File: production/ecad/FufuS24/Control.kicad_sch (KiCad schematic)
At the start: 28 parts, among them J14 691137710004, J15 691137710004, J16 691137710004, J2 Conn_01x02, U1 RP2040, U2 W25Q128JVS

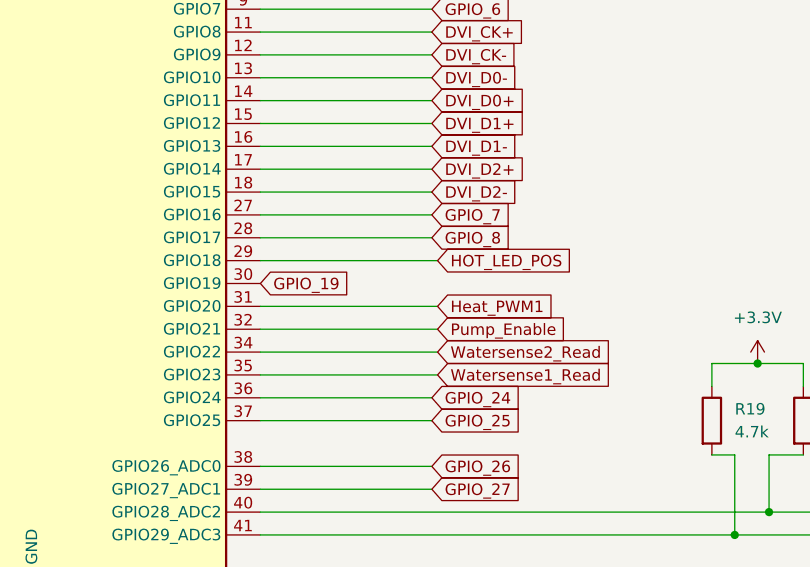
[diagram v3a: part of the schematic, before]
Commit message: changes
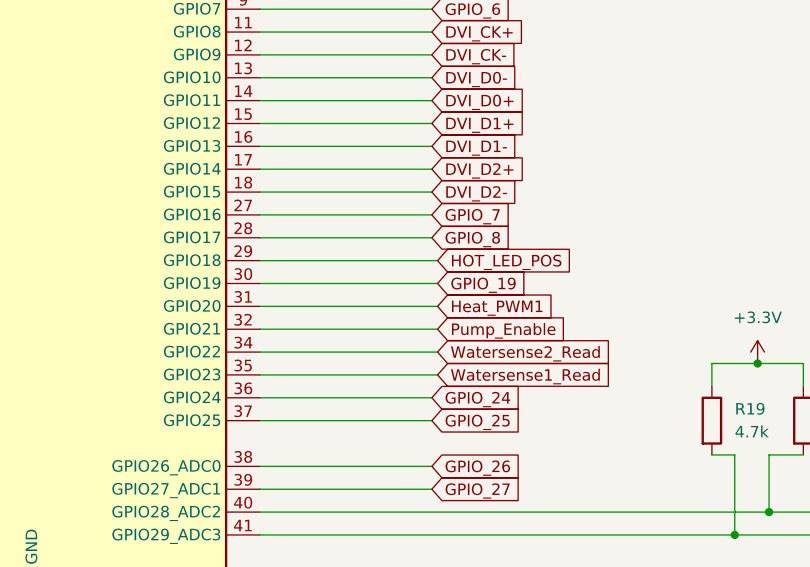
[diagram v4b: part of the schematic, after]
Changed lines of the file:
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@@
+    (stroke (width 0) (type default))
+  )
+  (wire (pts (xy 162.56 118.11) (xy 142.875 118.11))
     (stroke (width 0) (type default))
   )
@@
     )
   )
-  (global_label "GPIO_19" (shape input) (at 142.875 118.11 0) (fields_autoplaced)
-    (effects (font (size 1.27 1.27)) (justify left))
-    (property "Intersheetrefs" "${INTERSHEET_REFS}" (at 153.7221 118.11 0)
-      (effects (font (size 1.27 1.27)) (justify left) hide)
-    )
+  (global_label "GPIO_19" (shape input) (at 162.56 118.11 0) (fields_autoplaced)
+    (effects (font (size 1.27 1.27)) (justify left))
+    (property "Intersheetrefs" "${INTERSHEET_REFS}" (at 173.4071 118.11 0)
+      (effects (font (size 1.27 1.27)) (justify left) hide)
+    )
